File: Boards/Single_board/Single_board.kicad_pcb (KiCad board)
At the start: 2 copper layers, 169.9 x 190.9 mm, 132 parts, among them J1 AUX_I2C_1, J2 AUX_I2C_2, J3 USB_C_Receptacle_USB2.0_16P, J4 ICSP, Q1 SI2306, Q10 SI2306, Q11 SI2306, Q12 SI2306, Q13 SI2306, Q14 SI2306, Q15 SI2306, Q2 SI2306, Q3 SI2306, Q4 SI2306, Q5 SI2306, Q6 SI2306, Q7 SI2306, Q8 SI2306, Q9 SI2306, SW1 +, SW10 5, SW11 2, SW12 9, SW13 PRO, SW14 6, SW15 3, SW16 CLR, SW17 ENTR, SW18 RSET, SW19 KEYREL, SW2 VERB, SW3 NOUN, SW4 0, SW5 7, SW6 -, SW7 4, SW8 1, SW9 8, U1 PCF8575, U2 ATmega328P-A, U3 CH340C

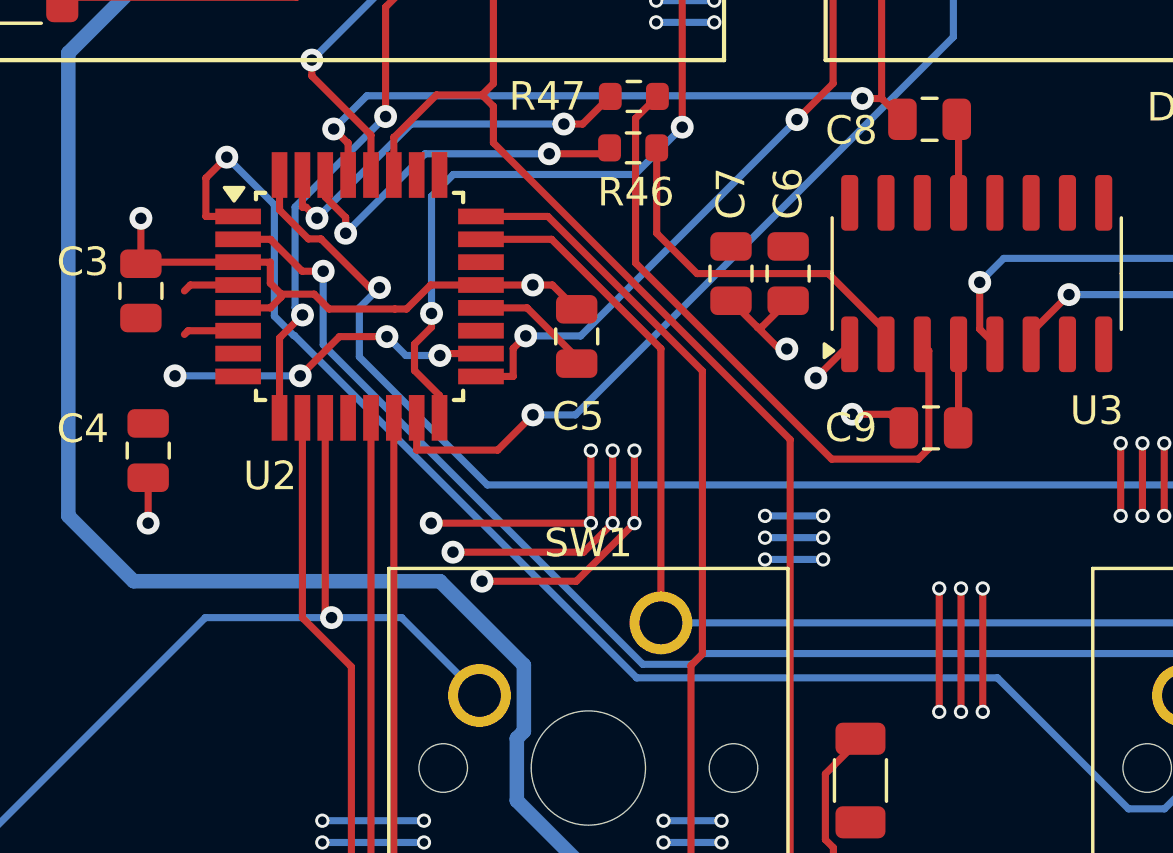
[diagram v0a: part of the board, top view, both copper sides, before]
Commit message: Better via placement
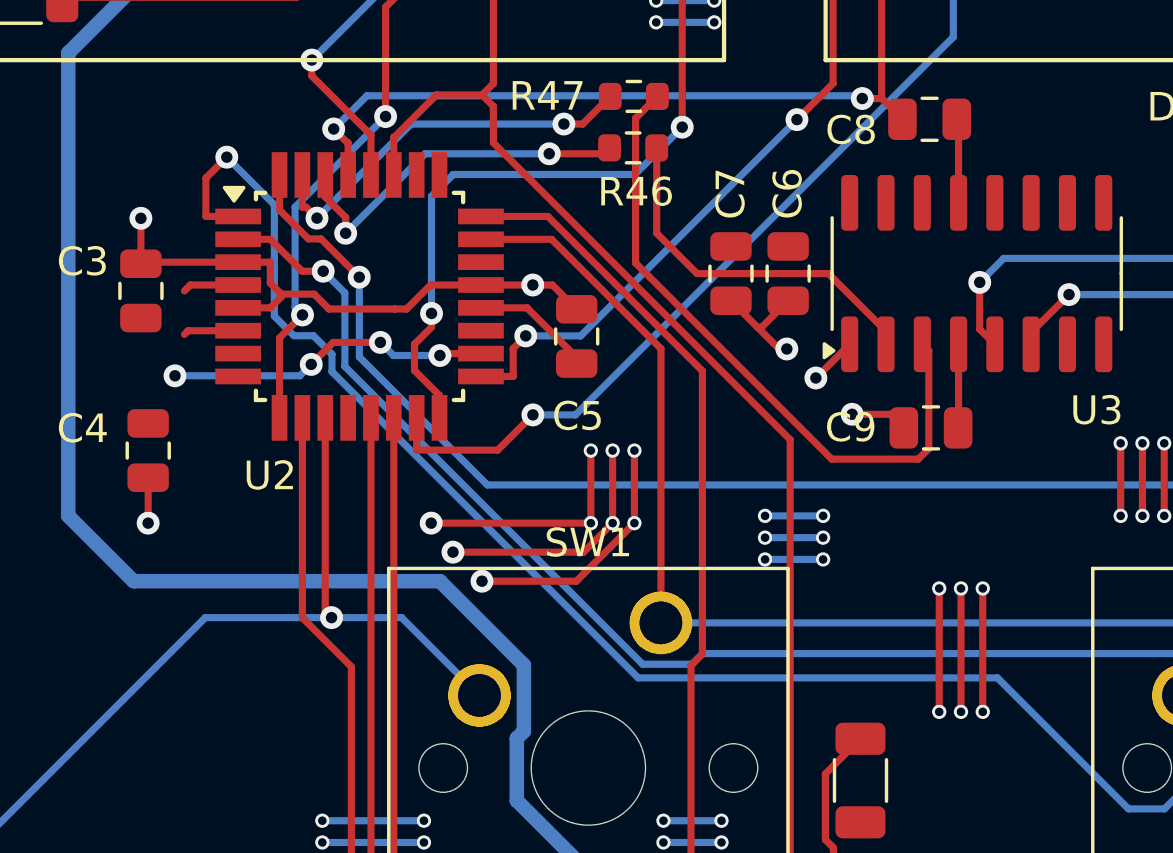
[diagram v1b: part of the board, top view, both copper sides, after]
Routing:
- net X4: track 221.1 -> 220.4 mm
